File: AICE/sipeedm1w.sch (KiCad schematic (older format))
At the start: 5 parts

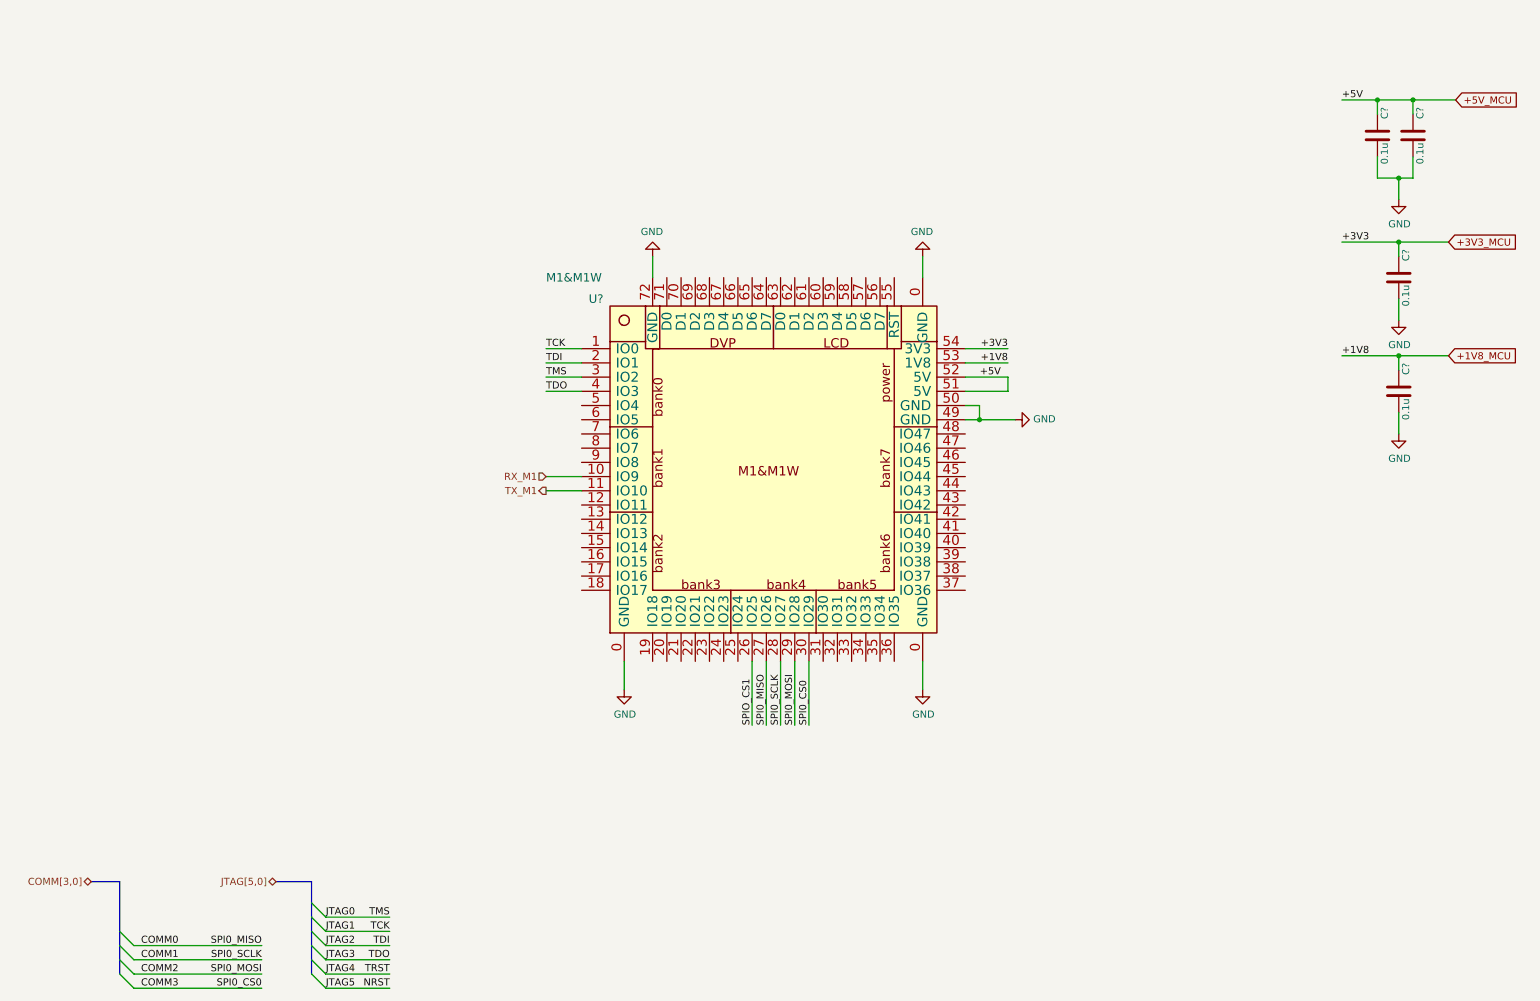
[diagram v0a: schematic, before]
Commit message: Add files via upload
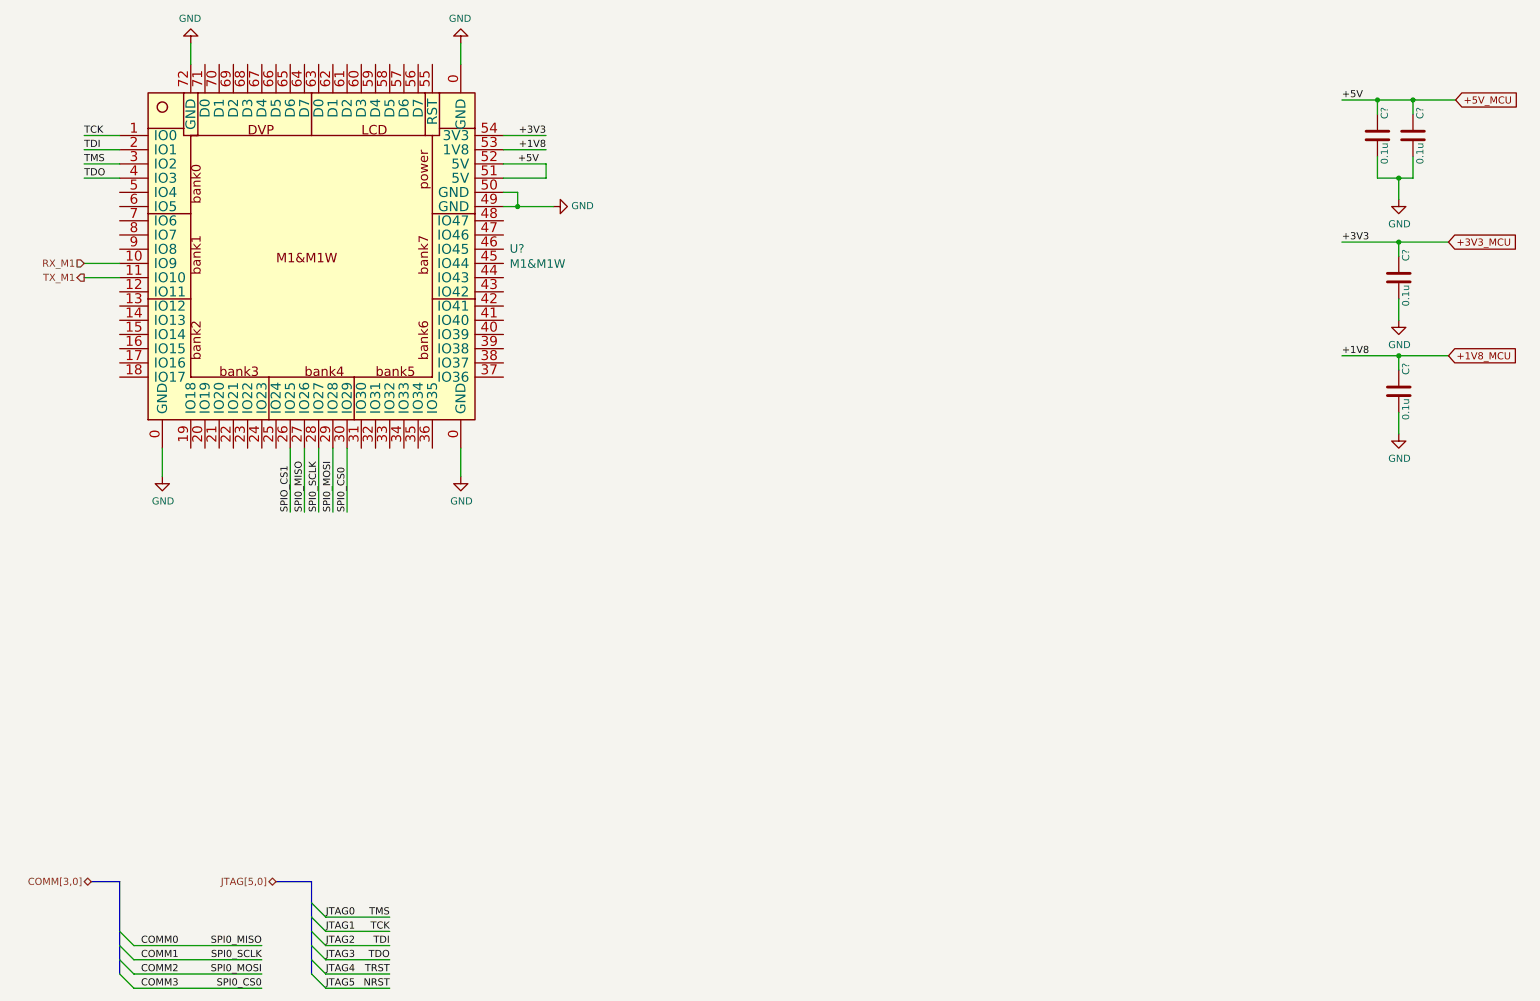
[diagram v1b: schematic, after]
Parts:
- removed U?: M1&M1W, symbol M1&M1w:M1&M1W
- added U?: M1&M1W, symbol M1&M1w:M1&M1W
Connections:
- net +1V8_MCU: now also U?.53 (1V8)
- net +3V3_MCU: now also U?.54 (3V3)
- net +5V_MCU: now also U?.51 (5V), U?.52 (5V)
- net COMM0: now also U?.27 (IO26)
- net COMM1: now also U?.28 (IO27)
- net COMM2: now also U?.29 (IO28)
- net COMM3: now also U?.30 (IO29)
- net GND: now also U?.0 (GND), U?.49 (GND), U?.50 (GND), U?.72 (GND)
- net JTAG0: now also U?.3 (IO2)
- net JTAG1: now also U?.1 (IO0)
- net JTAG2: now also U?.2 (IO1)
- net JTAG3: now also U?.4 (IO3)
- net RX_M1: now also U?.10 (IO9)
- net SPIO_CS1: now also U?.26 (IO25)
- net TX_M1: now also U?.11 (IO10)
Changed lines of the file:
@@
 Comment4 ""
 $EndDescr
-$Comp
-L M1&M1w:M1&M1W U?
-U 1 1 5E8295EC
-P 4750 2650
-F 0 "U?" H 4600 2700 60  0000 L CNN
-F 1 "M1&M1W" H 4300 2850 60  0000 L CNN
-F 2 "" H 4750 2650 60  0000 C CNN
-F 3 "" H 4750 2650 60  0000 C CNN
-	1    4750 2650
-	1    0    0    -1
-$EndComp
-Text Label 5750 5600 1    50   ~ 0
+Text Label 2500 4100 1    50   ~ 0
 SPIO_CS1
 Wire Wire Line
-	5750 5150 5750 5600
-Wire Wire Line
-	5850 5150 5850 5600
-Wire Wire Line
-	5950 5150 5950 5600
-Wire Wire Line
-	6050 5150 6050 5600
-Wire Wire Line
-	6150 5150 6150 5600
-Text Label 5850 5600 1    50   ~ 0
+	2500 3650 2500 4100
+Wire Wire Line
+	2600 3650 2600 4100
+Wire Wire Line
+	2700 3650 2700 4100
+Wire Wire Line
+	2800 3650 2800 4100
+Wire Wire Line
+	2900 3650 2900 4100
+Text Label 2600 4100 1    50   ~ 0
 SPI0_MISO
-Text Label 5950 5600 1    50   ~ 0
+Text Label 2700 4100 1    50   ~ 0
 SPI0_SCLK
-Text Label 6050 5600 1    50   ~ 0
+Text Label 2800 4100 1    50   ~ 0
 SPI0_MOSI
-Text Label 6150 5600 1    50   ~ 0
+Text Label 2900 4100 1    50   ~ 0
 SPI0_CS0
 Entry Wire Line
@@
 Text HLabel 1100 6700 0    50   BiDi ~ 0
 COMM[3,0]
-Text Label 4300 2950 0    50   ~ 0
+Text Label 1050 1450 0    50   ~ 0
 TCK
-Text Label 4300 3050 0    50   ~ 0
+Text Label 1050 1550 0    50   ~ 0
 TDI
-Text Label 4300 3150 0    50   ~ 0
+Text Label 1050 1650 0    50   ~ 0
 TMS
-Text Label 4300 3250 0    50   ~ 0
+Text Label 1050 1750 0    50   ~ 0
 TDO
 Wire Wire Line
-	4300 2950 4550 2950
-Wire Wire Line
-	4300 3050 4550 3050
-Wire Wire Line
-	4300 3150 4550 3150
-Wire Wire Line
-	4300 3250 4550 3250
+	1050 1450 1300 1450
+Wire Wire Line
+	1050 1550 1300 1550
+Wire Wire Line
+	1050 1650 1300 1650
+Wire Wire Line
+	1050 1750 1300 1750
 Wire Bus Line
 	2650 6700 2400 6700
@@
 NRST
 Wire Wire Line
-	4550 3850 4300 3850
-Wire Wire Line
-	4550 3950 4300 3950
-Text HLabel 4300 3850 0    50   Input ~ 0
+	1300 2350 1050 2350
+Wire Wire Line
+	1300 2450 1050 2450
+Text HLabel 1050 2350 0    50   Input ~ 0
 RX_M1
-Text HLabel 4300 3950 0    50   Output ~ 0
+Text HLabel 1050 2450 0    50   Output ~ 0
 TX_M1
 $Comp
 L power:GND #PWR?
 U 1 1 5EB07062
-P 6950 5350
-F 0 "#PWR?" H 6950 5100 50  0001 C CNN
-F 1 "GND" H 6955 5177 50  0000 C CNN
-F 2 "" H 6950 5350 50  0001 C CNN
-F 3 "" H 6950 5350 50  0001 C CNN
-	1    6950 5350
+P 3700 3850
+F 0 "#PWR?" H 3700 3600 50  0001 C CNN
+F 1 "GND" H 3705 3677 50  0000 C CNN
+F 2 "" H 3700 3850 50  0001 C CNN
+F 3 "" H 3700 3850 50  0001 C CNN
+	1    3700 3850
 	1    0    0    -1
 $EndComp
@@
 L power:GND #PWR?
 U 1 1 5EB07767
-P 4850 5350
-F 0 "#PWR?" H 4850 5100 50  0001 C CNN
-F 1 "GND" H 4855 5177 50  0000 C CNN
-F 2 "" H 4850 5350 50  0001 C CNN
-F 3 "" H 4850 5350 50  0001 C CNN
-	1    4850 5350
+P 1600 3850
+F 0 "#PWR?" H 1600 3600 50  0001 C CNN
+F 1 "GND" H 1605 3677 50  0000 C CNN
+F 2 "" H 1600 3850 50  0001 C CNN
+F 3 "" H 1600 3850 50  0001 C CNN
+	1    1600 3850
 	1    0    0    -1
 $EndComp
@@
 L power:GND #PWR?
 U 1 1 5EB07C18
-P 6950 2300
-F 0 "#PWR?" H 6950 2050 50  0001 C CNN
-F 1 "GND" H 6955 2127 50  0000 C CNN
-F 2 "" H 6950 2300 50  0001 C CNN
-F 3 "" H 6950 2300 50  0001 C CNN
-	1    6950 2300
+P 3700 800
+F 0 "#PWR?" H 3700 550 50  0001 C CNN
+F 1 "GND" H 3705 627 50  0000 C CNN
+F 2 "" H 3700 800 50  0001 C CNN
+F 3 "" H 3700 800 50  0001 C CNN
+	1    3700 800
 	-1   0    0    1
 $EndComp
@@
 L power:GND #PWR?
 U 1 1 5EB09351
-P 7600 3450
-F 0 "#PWR?" H 7600 3200 50  0001 C CNN
-F 1 "GND" V 7605 3322 50  0000 R CNN
-F 2 "" H 7600 3450 50  0001 C CNN
-F 3 "" H 7600 3450 50  0001 C CNN
-	1    7600 3450
+P 4350 1950
+F 0 "#PWR?" H 4350 1700 50  0001 C CNN
+F 1 "GND" V 4355 1822 50  0000 R CNN
+F 2 "" H 4350 1950 50  0001 C CNN
+F 3 "" H 4350 1950 50  0001 C CNN
+	1    4350 1950
 	0    -1   -1   0
 $EndComp
 Wire Wire Line
-	7250 3450 7350 3450
-Wire Wire Line
-	7250 3350 7350 3350
-Wire Wire Line
-	7350 3350 7350 3450
-Connection ~ 7350 3450
-Wire Wire Line
-	7350 3450 7600 3450
-Wire Wire Line
-	6950 5350 6950 5150
-Wire Wire Line
-	4850 5150 4850 5350
-Wire Wire Line
-	6950 2450 6950 2300
+	4000 1950 4100 1950
+Wire Wire Line
+	4000 1850 4100 1850
+Wire Wire Line
+	4100 1850 4100 1950
+Connection ~ 4100 1950
+Wire Wire Line
+	4100 1950 4350 1950
+Wire Wire Line
+	3700 3850 3700 3650
+Wire Wire Line
+	1600 3650 1600 3850
+Wire Wire Line
+	3700 950  3700 800
 $Comp
 L Device:C C?
@@
 +5V_MCU
 Wire Wire Line
-	7250 3150 7550 3150
-Wire Wire Line
-	7550 3150 7550 3250
-Wire Wire Line
-	7550 3250 7250 3250
-Text Label 7500 3150 2    50   ~ 0
+	4000 1650 4300 1650
+Wire Wire Line
+	4300 1650 4300 1750
+Wire Wire Line
+	4300 1750 4000 1750
+Text Label 4250 1650 2    50   ~ 0
 +5V
-Text Label 7550 3050 2    50   ~ 0
+Text Label 4300 1550 2    50   ~ 0
 +1V8
-Text Label 7550 2950 2    50   ~ 0
+Text Label 4300 1450 2    50   ~ 0
 +3V3
 Wire Wire Line
-	7250 2950 7550 2950
-Wire Wire Line
-	7250 3050 7550 3050
+	4000 1450 4300 1450
+Wire Wire Line
+	4000 1550 4300 1550
 Connection ~ 10150 1200
 Wire Wire Line
@@
 L power:GND #PWR?
 U 1 1 5EB59EFD
-P 5050 2300
-F 0 "#PWR?" H 5050 2050 50  0001 C CNN
-F 1 "GND" H 5055 2127 50  0000 C CNN
-F 2 "" H 5050 2300 50  0001 C CNN
-F 3 "" H 5050 2300 50  0001 C CNN
-	1    5050 2300
-	-1   0    0    1
-$EndComp
-Wire Wire Line
-	5050 2450 5050 2300
+P 1800 800
+F 0 "#PWR?" H 1800 550 50  0001 C CNN
+F 1 "GND" H 1805 627 50  0000 C CNN
+F 2 "" H 1800 800 50  0001 C CNN
+F 3 "" H 1800 800 50  0001 C CNN
+	1    1800 800
+	-1   0    0    1
+$EndComp
+Wire Wire Line
+	1800 950  1800 800
+$Comp
+L M1&M1w:M1&M1W U?
+U 1 1 5E97DB3F
+P 1500 1150
+F 0 "U?" H 4044 53  60  0000 L CNN
+F 1 "M1&M1W" H 4044 -53 60  0000 L CNN
+F 2 "" H 1500 1150 60  0000 C CNN
+F 3 "" H 1500 1150 60  0000 C CNN
+	1    1500 1150
+	1    0    0    -1
+$EndComp
 Wire Bus Line
 	1300 6700 1300 7350
